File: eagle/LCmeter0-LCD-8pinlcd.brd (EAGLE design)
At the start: 58.4 x 48.2 mm, 27 parts, among them IC1 PIC16F876A-X/SP, K2 DS2Y, Q1 20MHz, Q2 BC548, SW1 SPST, X1 FREQ, X2 L/C

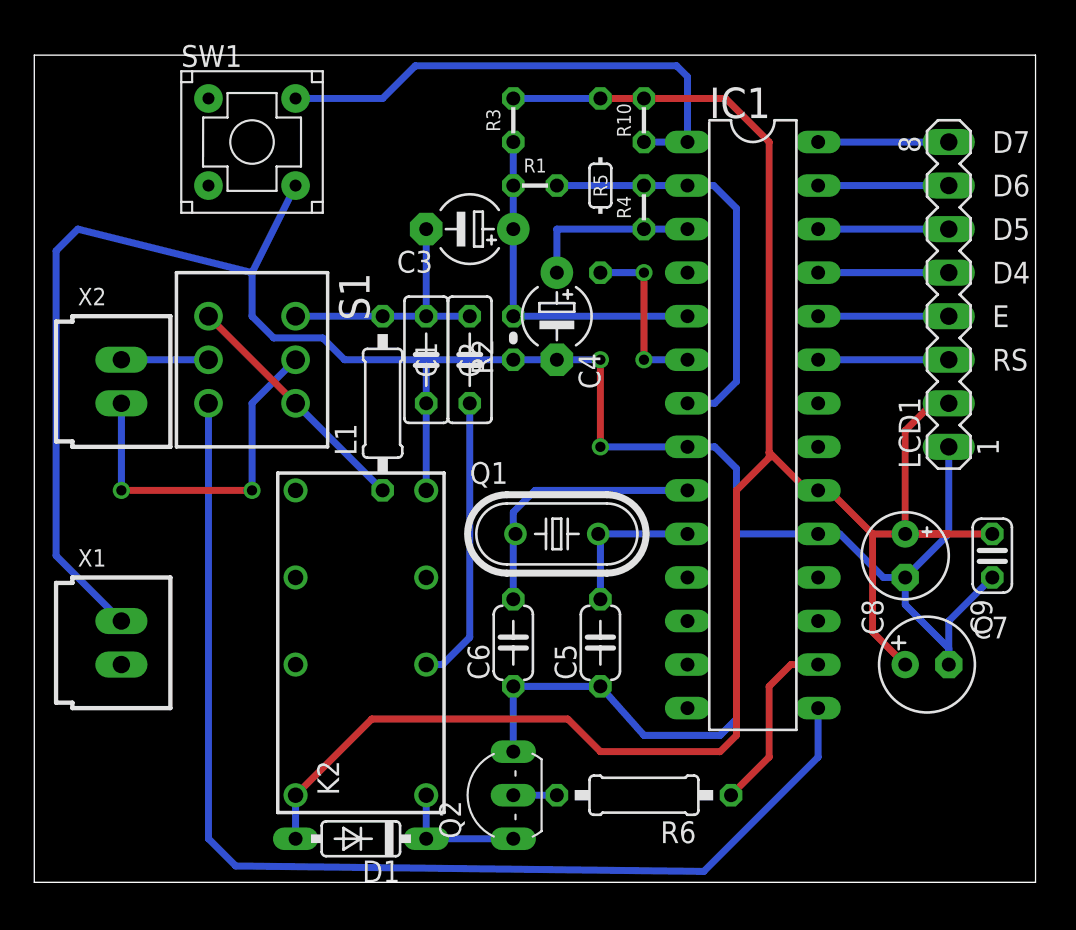
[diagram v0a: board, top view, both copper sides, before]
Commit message: ...
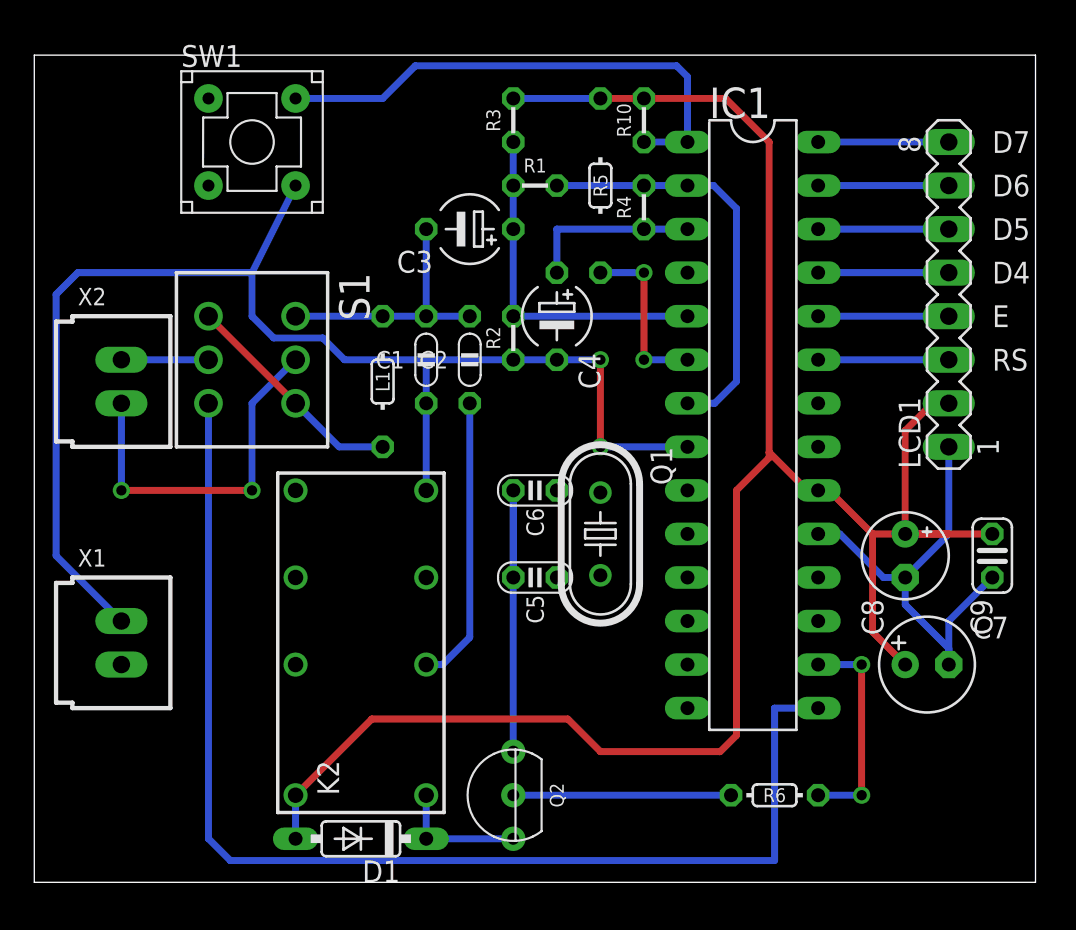
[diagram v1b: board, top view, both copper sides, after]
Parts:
- C1, C2: device rcl:C050-025X075 -> c:C050-020X036
- C3, C4: device rcl:E5-4 -> c:E5-4
- C5, C6: device rcl:C050-024X044 -> c:C025-020X036
- L1: device rcl:0207/10 -> r:0202/7
- Q2: value BC548 -> BC547CBE; device transistor-npn:TO92-EBC -> t:TO92-CBE
- R2: device resistor:0204V -> r:0202/2V
- R6: device rcl:0207/10 -> r:0202/5
- moved C6 8.98 mm to (29.2, 22.9)
- moved R6 7.62 mm to (43.2, 5.08), turned to 90 degrees
- moved C5 5.39 mm to (29.2, 17.8)
- moved Q1 2.54 mm to (33.0, 20.3), turned to 270 degrees
- moved L1 1.27 mm to (20.3, 29.2), turned to 0 degrees
- moved Q2 1.27 mm to (27.9, 5.08)
- turned C1 to 0 degrees
- turned C2 to 0 degrees
- turned R2 to 0 degrees
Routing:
- net GND: track 151.1 -> 127.3 mm
- net OSC1: track 15.9 -> 0.00 mm
- net N$5: track 2.54 -> 12.7 mm
- net OSC2: track 8.89 -> 0.00 mm
- net /LC: track 67.2 -> 70.4 mm
- net RC5: track 10.7 -> 12.7 mm, vias 0 -> 2
- net N$7: track 14.4 -> 13.3 mm
